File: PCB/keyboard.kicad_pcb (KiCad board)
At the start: 2 copper layers, 30 parts, among them SW1 SW_Push, SW11 RotaryEncoder, SW2 SW_Push, SW3 SW_Push, SW4 SW_Push, SW5 SW_Push, SW6 SW_Push, SW7 SW_Push, SW8 SW_Push, SW9 SW_Push, U1 XIAO-RP2040-DIP, U2 74AHC1G125

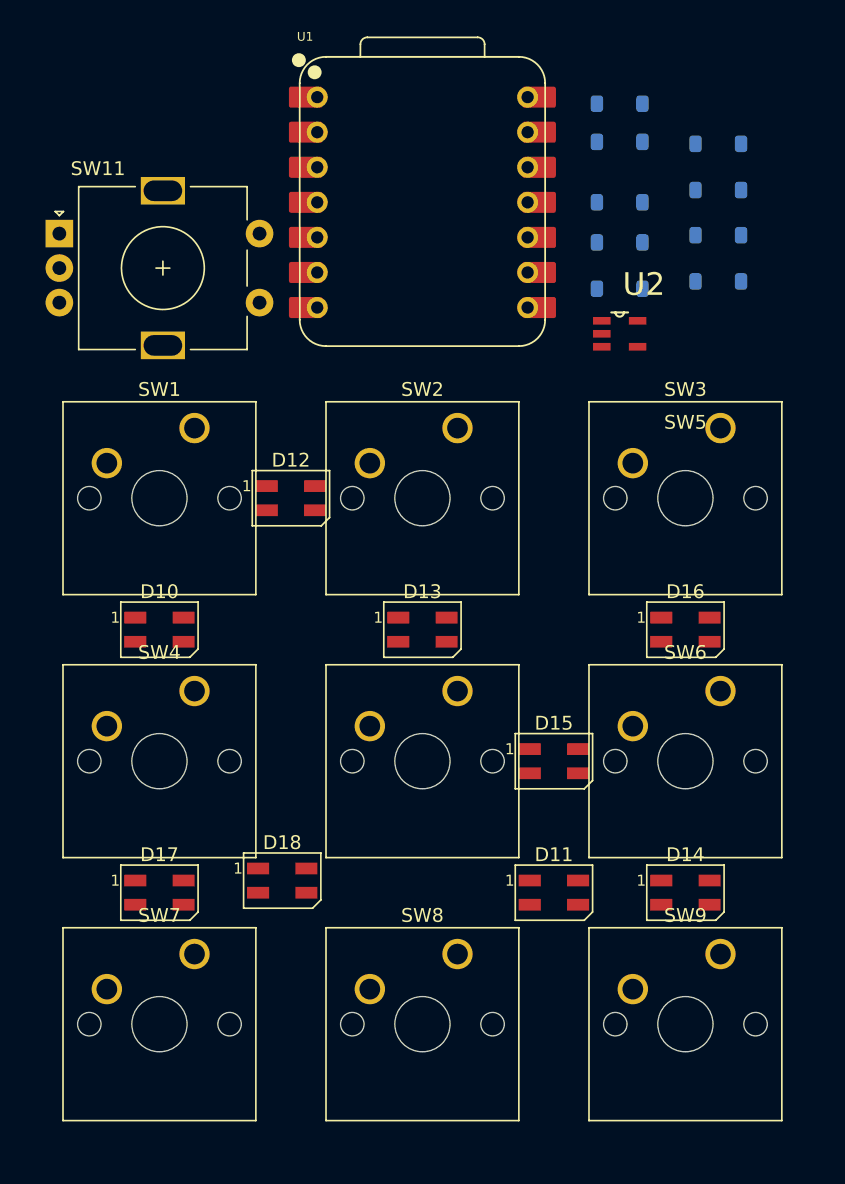
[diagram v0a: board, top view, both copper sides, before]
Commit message: final?
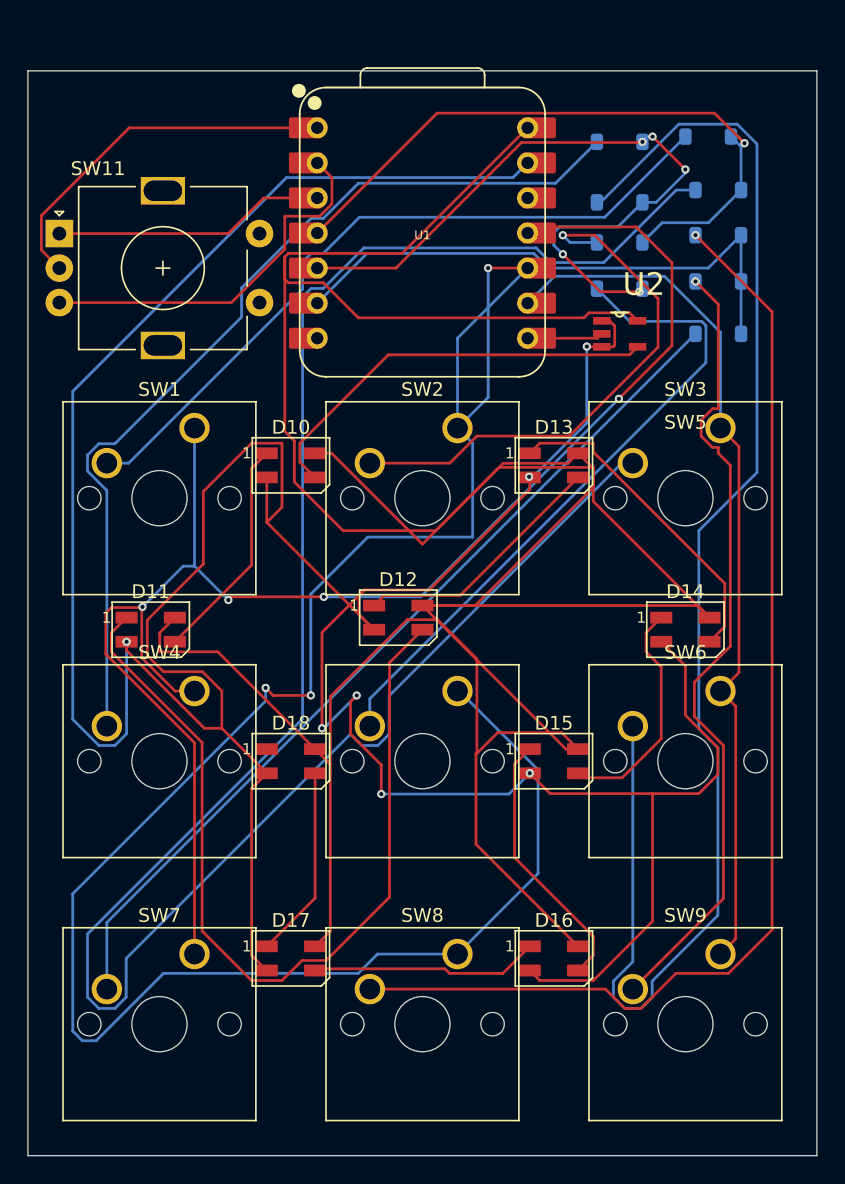
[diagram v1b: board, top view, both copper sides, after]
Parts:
- moved D11 34.9 mm to (80.3, 54.8)
- moved D16 25.6 mm to (109.5, 78.6)
- moved D14 19.0 mm to (119.1, 54.8)
- moved D3 18.1 mm to (121.4, 33.3)
- moved D10 15.2 mm to (90.5, 42.9)
- moved D13 15.2 mm to (109.5, 42.9)
- moved D12 11.6 mm to (98.3, 53.9)
- moved D17 10.6 mm to (90.5, 78.6)
- moved D18 8.67 mm to (90.5, 64.3)
- moved D1 7.99 mm to (120.7, 19.1)
- moved D8 7.53 mm to (114.3, 23.8)
- moved D6 6.62 mm to (121.4, 26.2)
- moved U1 2.22 mm to (100.0, 26.0)
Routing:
- net GND: track 0.00 -> 271.3 mm, vias 0 -> 7
- net +5V: track 0.00 -> 270.0 mm
- net Net-(D7-A): track 0.00 -> 149.9 mm
- net Net-(U1-GPIO4/MISO): track 0.00 -> 147.1 mm, vias 0 -> 3
- net Net-(U1-GPIO3/MOSI): track 0.00 -> 114.5 mm, vias 0 -> 4
- net Net-(D8-A): track 0.00 -> 104.3 mm
- net Net-(D6-A): track 0.00 -> 84.7 mm, vias 0 -> 1
- net Net-(D2-A): track 0.00 -> 67.7 mm
- net Net-(D3-A): track 0.00 -> 65.1 mm
- net Net-(D11-DOUT): track 0.00 -> 63.8 mm
- net Net-(U1-GPIO2/SCK): track 0.00 -> 63.5 mm
- net Net-(D9-A): track 0.00 -> 58.5 mm, vias 0 -> 1
- net Net-(D1-A): track 0.00 -> 52.9 mm
- net Net-(D2-K): track 0.00 -> 51.7 mm, vias 0 -> 5
- net Net-(D1-K): track 0.00 -> 49.5 mm, vias 0 -> 1
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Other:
- board outline added: 57.2 x 78.6 mm
